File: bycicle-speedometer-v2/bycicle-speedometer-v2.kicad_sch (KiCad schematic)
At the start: 25 parts, among them J1 Conn_01x02_Pin, J2 Conn_01x02_Pin, J3 Conn_01x02_Pin, SW1 SW_Push_Dual, U1 ESP-12E, U2 AMS1117-3.3

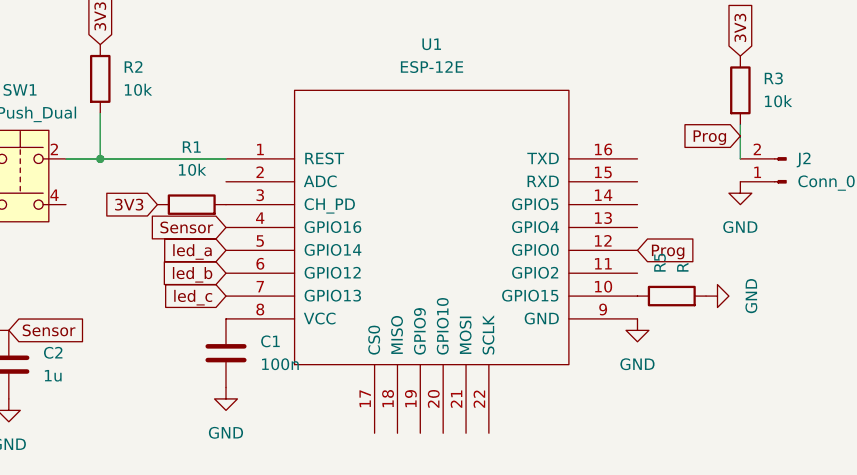
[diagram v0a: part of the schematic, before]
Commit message: edited schematics
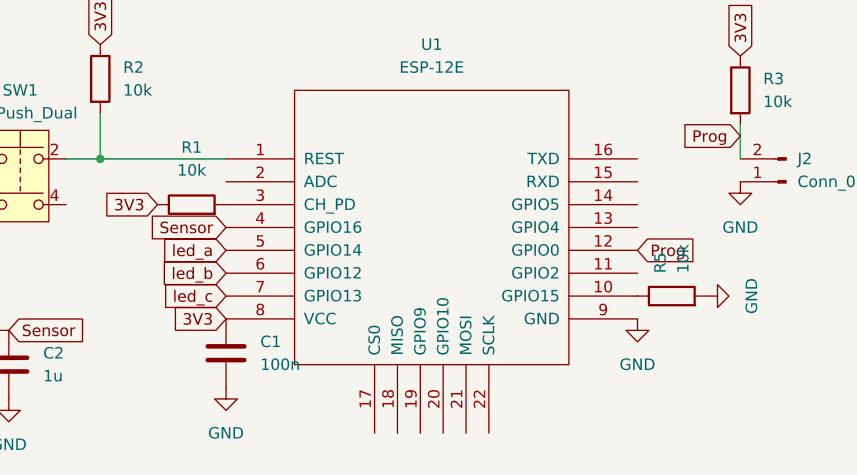
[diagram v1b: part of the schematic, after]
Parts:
- R5: value R -> 10k
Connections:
- net 3V3: now also C1.1, U1.8 (VCC)
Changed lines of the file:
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@@
+		)
+	)
+	(global_label "3V3"
+		(shape input)
+		(at 116.84 101.6 180)
+		(fields_autoplaced yes)
+		(effects
+			(font
+				(size 1.27 1.27)
+			)
+			(justify right)
+		)
+		(property "Intersheetrefs" "${INTERSHEET_REFS}"
+			(at 110.3472 101.6 0)
+			(effects
+				(font
+					(size 1.27 1.27)
+				)
+				(justify right)
+				(hide yes)
+			)
 		)
 	)
@@
 			)
 		)
-		(property "Value" "R"
+		(property "Value" "10k	"
 			(at 167.6399 96.52 0)
 			(effects
